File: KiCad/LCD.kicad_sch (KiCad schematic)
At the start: 4 parts

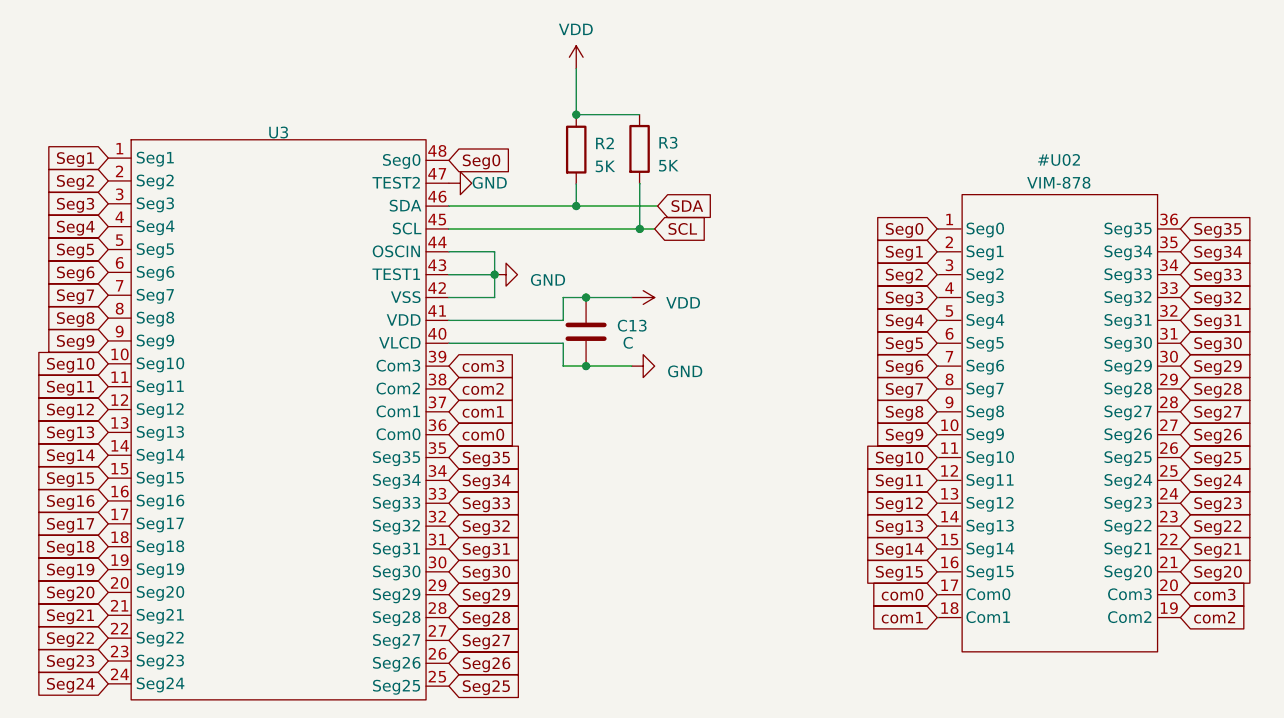
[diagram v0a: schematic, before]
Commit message: Ki cad schematic update.
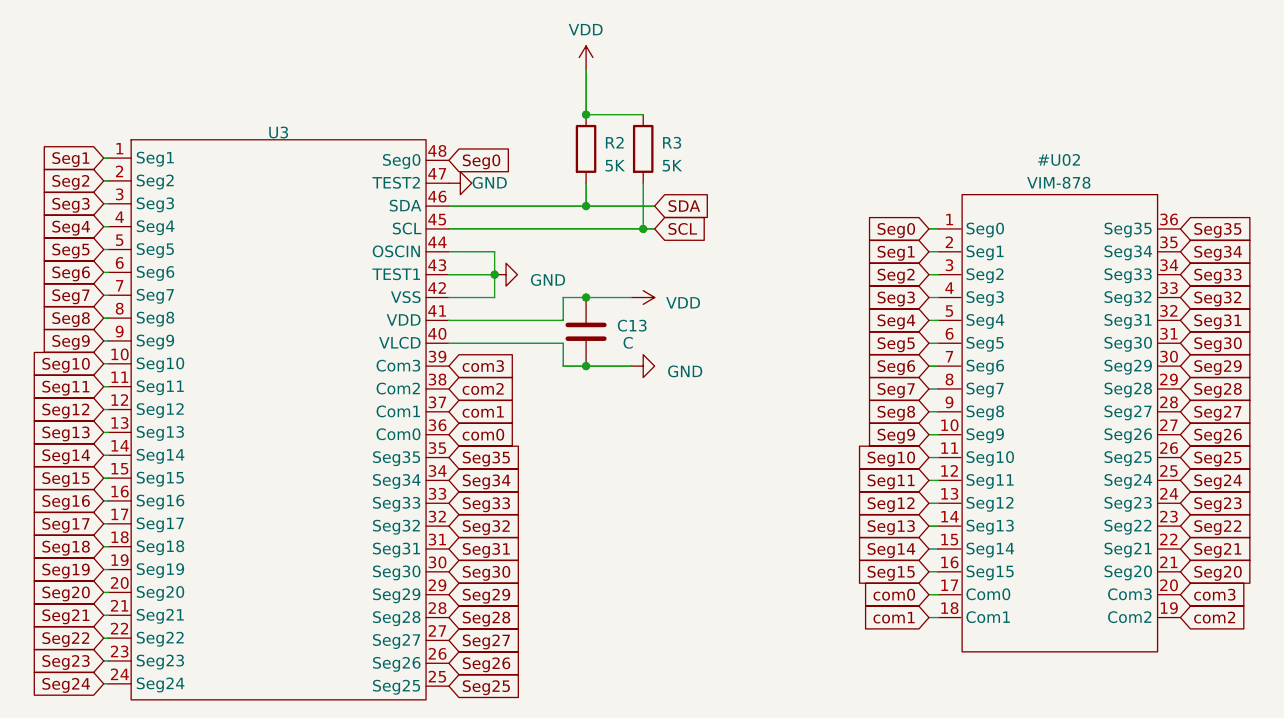
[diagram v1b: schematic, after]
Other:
- moved on the sheet: R2
